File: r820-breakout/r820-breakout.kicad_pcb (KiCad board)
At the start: 2 copper layers, 30.5 x 54.6 mm, 18 parts, among them J1 Conn_Coaxial, J2 Conn_01x10, J3 Conn_01x02, J4 Conn_01x02, U1 R820T, Y1 16MHz CL=16pF

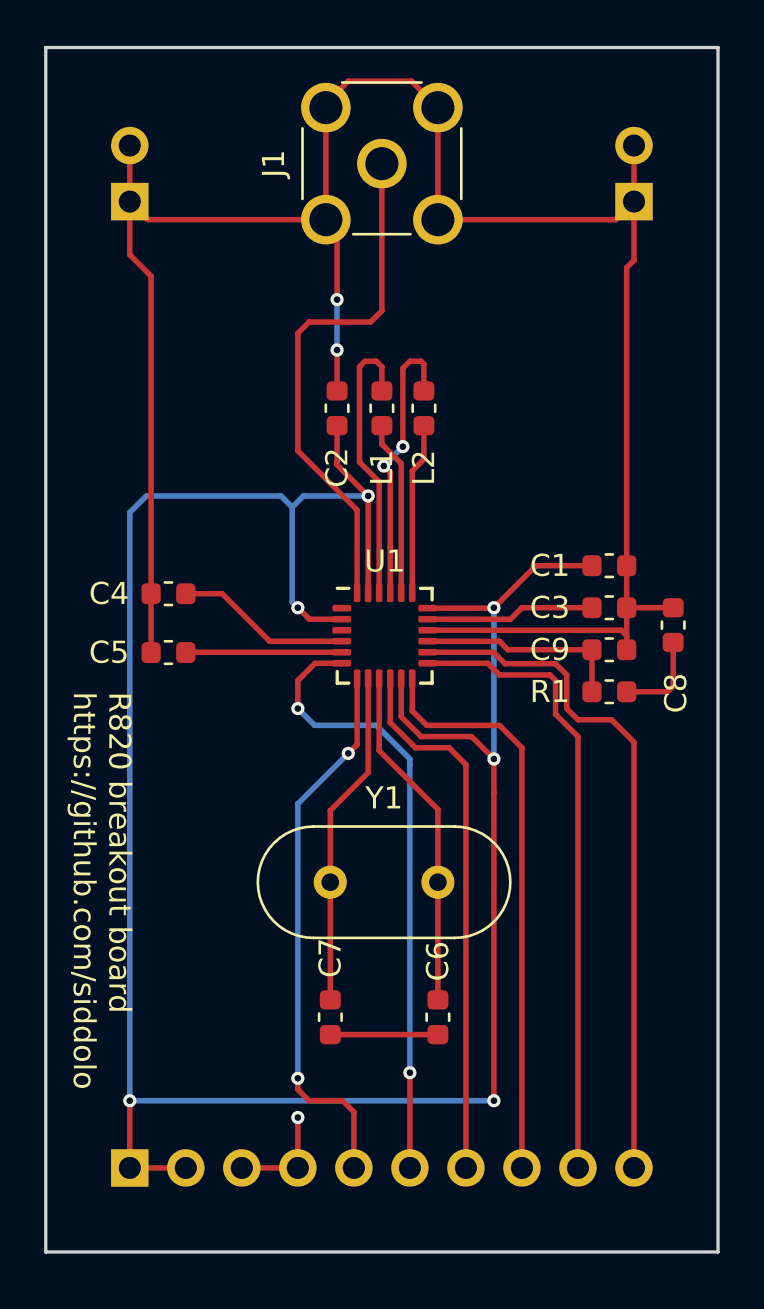
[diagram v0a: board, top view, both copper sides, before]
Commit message: Heavily reworked.
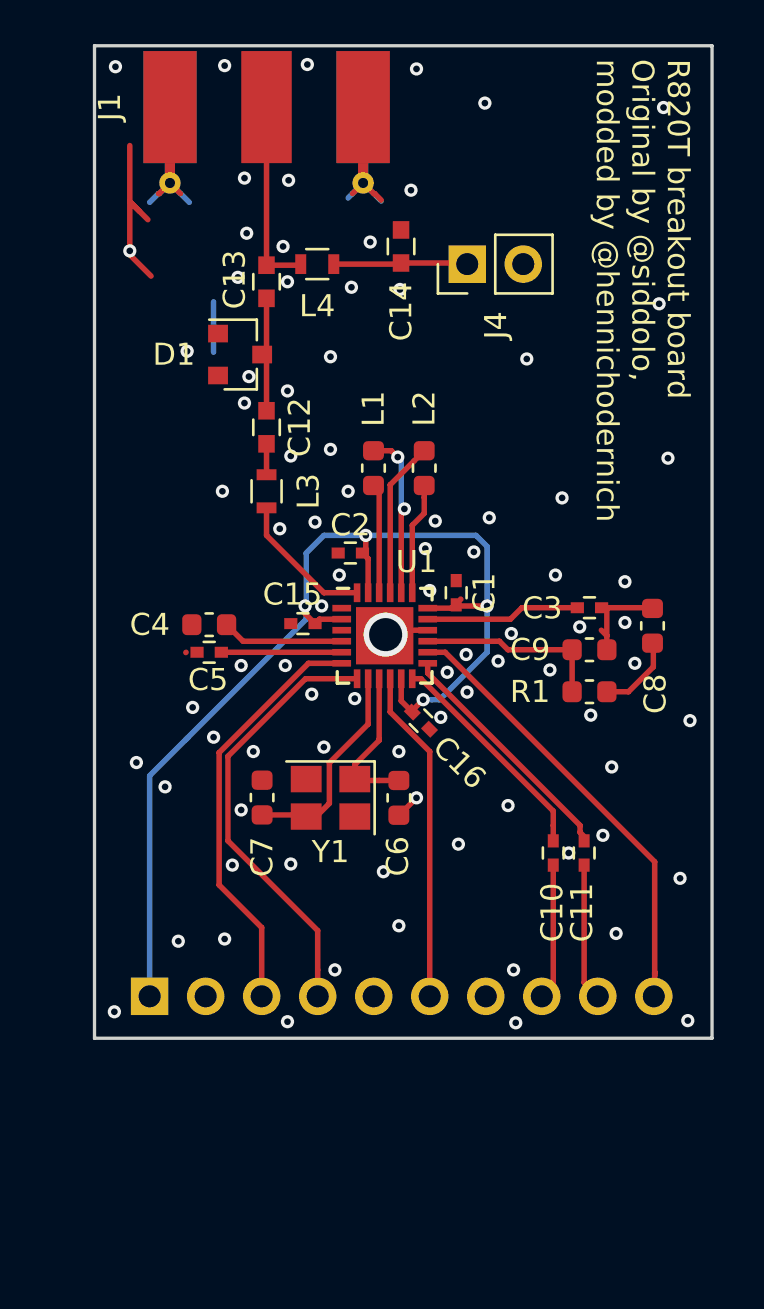
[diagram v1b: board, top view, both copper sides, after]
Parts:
- removed J3: Conn_01x02, Connector_PinHeader_2.54mm:PinHeader_1x02_P2.54mm_Vertical
- added C10: C, Capacitors_SMD:C_0402, F.Cu at (120.8, 105.1)
- added C11: C, Capacitors_SMD:C_0402, F.Cu at (122.2, 105.1)
- added C12: 330p, Capacitors_SMD:C_0603, F.Cu at (107.8, 85.8)
- added C13: 10n, Capacitors_SMD:C_0603, F.Cu at (107.8, 79.2)
- added C14: 100n, Capacitors_SMD:C_0603, F.Cu at (113.9, 77.6)
- added C15: 100nF, Capacitors_SMD:C_0402, F.Cu at (109.5, 94.7)
- added C16: 100nF, Capacitors_SMD:C_0402, F.Cu at (114.8, 99.1)
- added D1: BAV99, TO_SOT_Packages_SMD:SOT-23, F.Cu at (106.6, 82.5)
- added L3: 8.2n, Inductors_SMD:L_0603, F.Cu at (107.8, 88.7)
- added L4: 180n, Inductors_SMD:L_0603, F.Cu at (110.1, 78.4)
- C1, C2, C3, C5: footprint Capacitor_SMD:C_0603_1608Metric -> Capacitors_SMD:C_0402
- J1: footprint Connector_Coaxial:SMA_Molex_73251-2200_Horizontal -> Connectors_Molex:Molex_SMA_Jack_Edge_Mount
- J4: moved to F.Cu
- U1: footprint Sensor_Motion:InvenSense_QFN-24_4x4mm_P0.5mm -> Housings_DFN_QFN:QFN-24-1EP_4x4mm_Pitch0.5mm
- Y1: value 16MHz CL=16pF -> Crystal_GND24; footprint Crystal:Crystal_HC49-4H_Vertical -> Crystals:Crystal_SMD_TXC_7M-4pin_3.2x2.5mm
- moved C7 10.4 mm to (107.6, 102.6), turned to 90 degrees
- moved C6 10.1 mm to (113.8, 102.6)
- moved J4 8.07 mm to (116.9, 78.4), turned to 90 degrees
- moved J2 7.83 mm to (102.5, 111.6)
- moved C1 7.05 mm to (116.4, 93.3), turned to 270 degrees
- moved C2 6.59 mm to (111.6, 91.5), turned to 0 degrees
- moved Y1 6.19 mm to (110.7, 102.6)
- moved J1 5.30 mm to (107.8, 73.0), turned to 270 degrees
- moved L1 2.74 mm to (112.7, 87.7), turned to 270 degrees
- moved L2 2.71 mm to (115.0, 87.7)
- moved C4 2.32 mm to (105.2, 94.8)
- moved C5 1.85 mm to (105.2, 96.0)
- moved C8 0.94 mm to (125.3, 94.8)
- moved C3 0.90 mm to (122.4, 94.0)
- moved C9 0.90 mm to (122.4, 95.9)
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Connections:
- J2 pad 2: VDD_3V -> GND
- J2 pad 3: GND -> T_SCL
- J2 pad 4: GND -> T_SDA
- J2 pad 5: T_SDA -> GND
- J2 pad 6: T_SCL -> T_CLK_Out
- J2 pad 7: T_CLK_Out -> GND
- J4 pad 1: GND -> Net-(C14-Pad2)
- U1 pad 1: (no net) -> Net-(U1-Pad1)
- U1 pad 12: T_IF_N -> Net-(C10-Pad1)
- U1 pad 13: T_IF_P -> Net-(C11-Pad1)
- U1 pad 24: T_RF_IN -> Net-(L3-Pad2)
- U1 pad 3: (no net) -> Net-(U1-Pad3)
- Y1 pad 2: Net-(C7-Pad1) -> GND
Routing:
- net GND: track 110.8 -> 25.7 mm, vias 3 -> 86
- net VDD_3V: track 112.6 -> 50.8 mm, vias 6 -> 4
- net T_IF_P: track 28.6 -> 6.01 mm
- net T_IF_N: track 26.2 -> 5.97 mm
- net T_RF_IN: track 23.8 -> 8.74 mm
- net Net-(C11-Pad1): track 0.00 -> 10.8 mm
- net T_IF_AGC: track 31.2 -> 20.5 mm
- net Net-(C10-Pad1): track 0.00 -> 10.0 mm
- net T_CLK_Out: track 24.5 -> 15.1 mm
- net Net-(C6-Pad1): track 15.7 -> 6.54 mm
- net T_SCL: track 28.1 -> 19.1 mm, vias 2 -> 0
- net Net-(L1-Pad2): track 12.9 -> 4.87 mm
- net Net-(L3-Pad2): track 0.00 -> 6.43 mm
- net Net-(C14-Pad2): track 0.00 -> 6.09 mm
- net Net-(L2-Pad2): track 13.0 -> 7.08 mm, vias 2 -> 0
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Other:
- board size 30.5 x 54.6 mm -> 28 x 45 mm
- net class Default: clearance 0.2 -> 0.15
- rule trace_clearance: 0.2 -> 0.15
- rule trace_min: 0.2 -> 0.15
- board text added: "R820T breakout board Original by @siddolo, modded by @hennichodernich"
- board text removed: "R820 breakout board https://github.com/siddolo"
